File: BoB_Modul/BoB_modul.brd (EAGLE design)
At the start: 27.9 x 40.6 mm, 12 parts

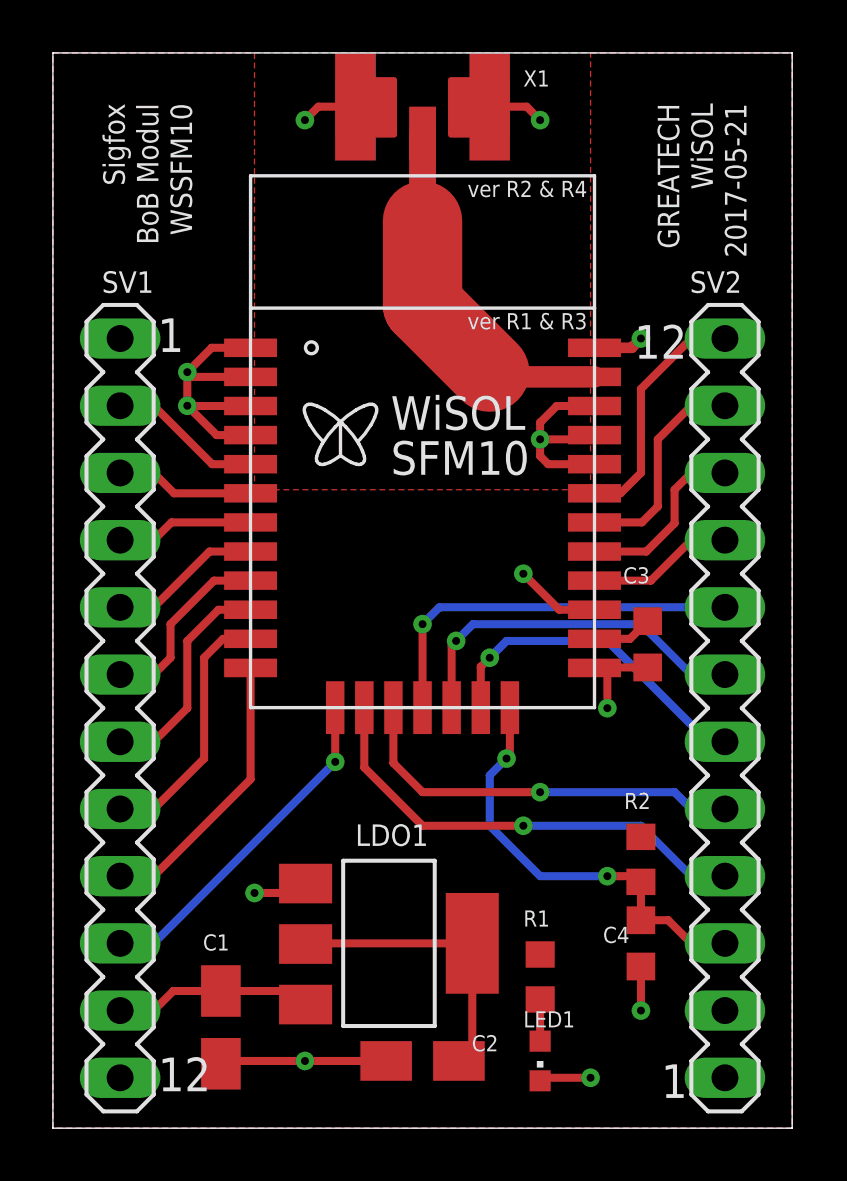
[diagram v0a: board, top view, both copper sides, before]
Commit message: make metric and nice, not yet finnished, work in progress
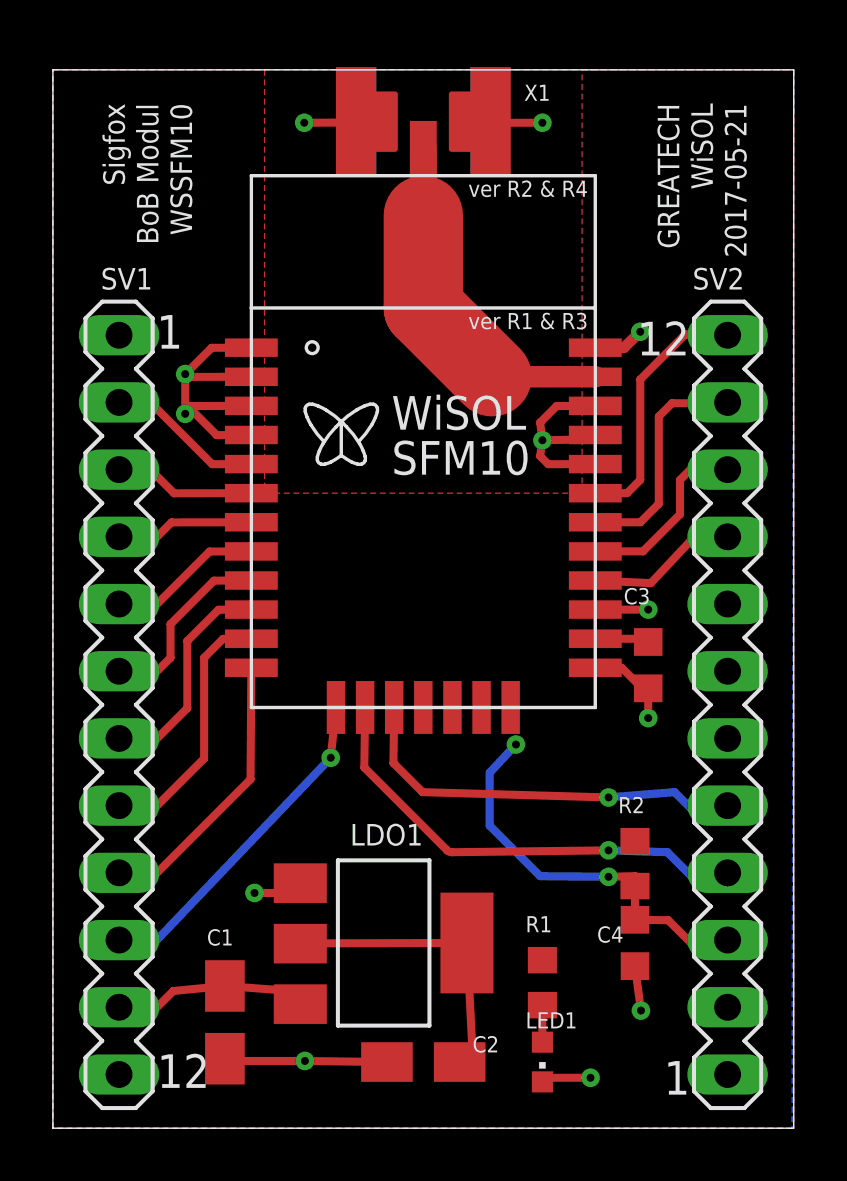
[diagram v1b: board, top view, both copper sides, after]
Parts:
- moved C3 0.79 mm to (22.5, 17.5)
- moved X1 0.54 mm to (14.0, 40.1)
- moved R2 0.28 mm to (22.0, 10.0)
- moved C1 0.24 mm to (6.50, 4.00)
- moved R1 0.23 mm to (18.5, 5.50)
- moved C4 0.23 mm to (22.0, 7.00)
- moved LDO1 0.20 mm to (12.5, 7.00)
- moved SV2 0.16 mm to (25.5, 16.0)
- moved SV1 0.13 mm to (2.50, 16.0)
- moved LED1 0.09 mm to (18.5, 2.50)
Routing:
- net DBG_DATA_RX_LED: track 14.8 -> 0.00 mm, vias 1 -> 0
- net DBG_CLK_TX_LED: track 13.8 -> 0.00 mm, vias 1 -> 0
- net DBG_EN_NC: track 12.8 -> 0.00 mm, vias 1 -> 0
- net /RST: track 16.4 -> 15.3 mm
- net GND: track 45.9 -> 45.1 mm
- net GPIO2: track 8.24 -> 8.81 mm
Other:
- board size 27.9 x 40.6 mm -> 28 x 40 mm
